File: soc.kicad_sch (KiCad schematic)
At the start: 10 parts, among them U1 STM32MP135AAFx, U2 STM32MP131AAEx, U3 ATSAMA5D21

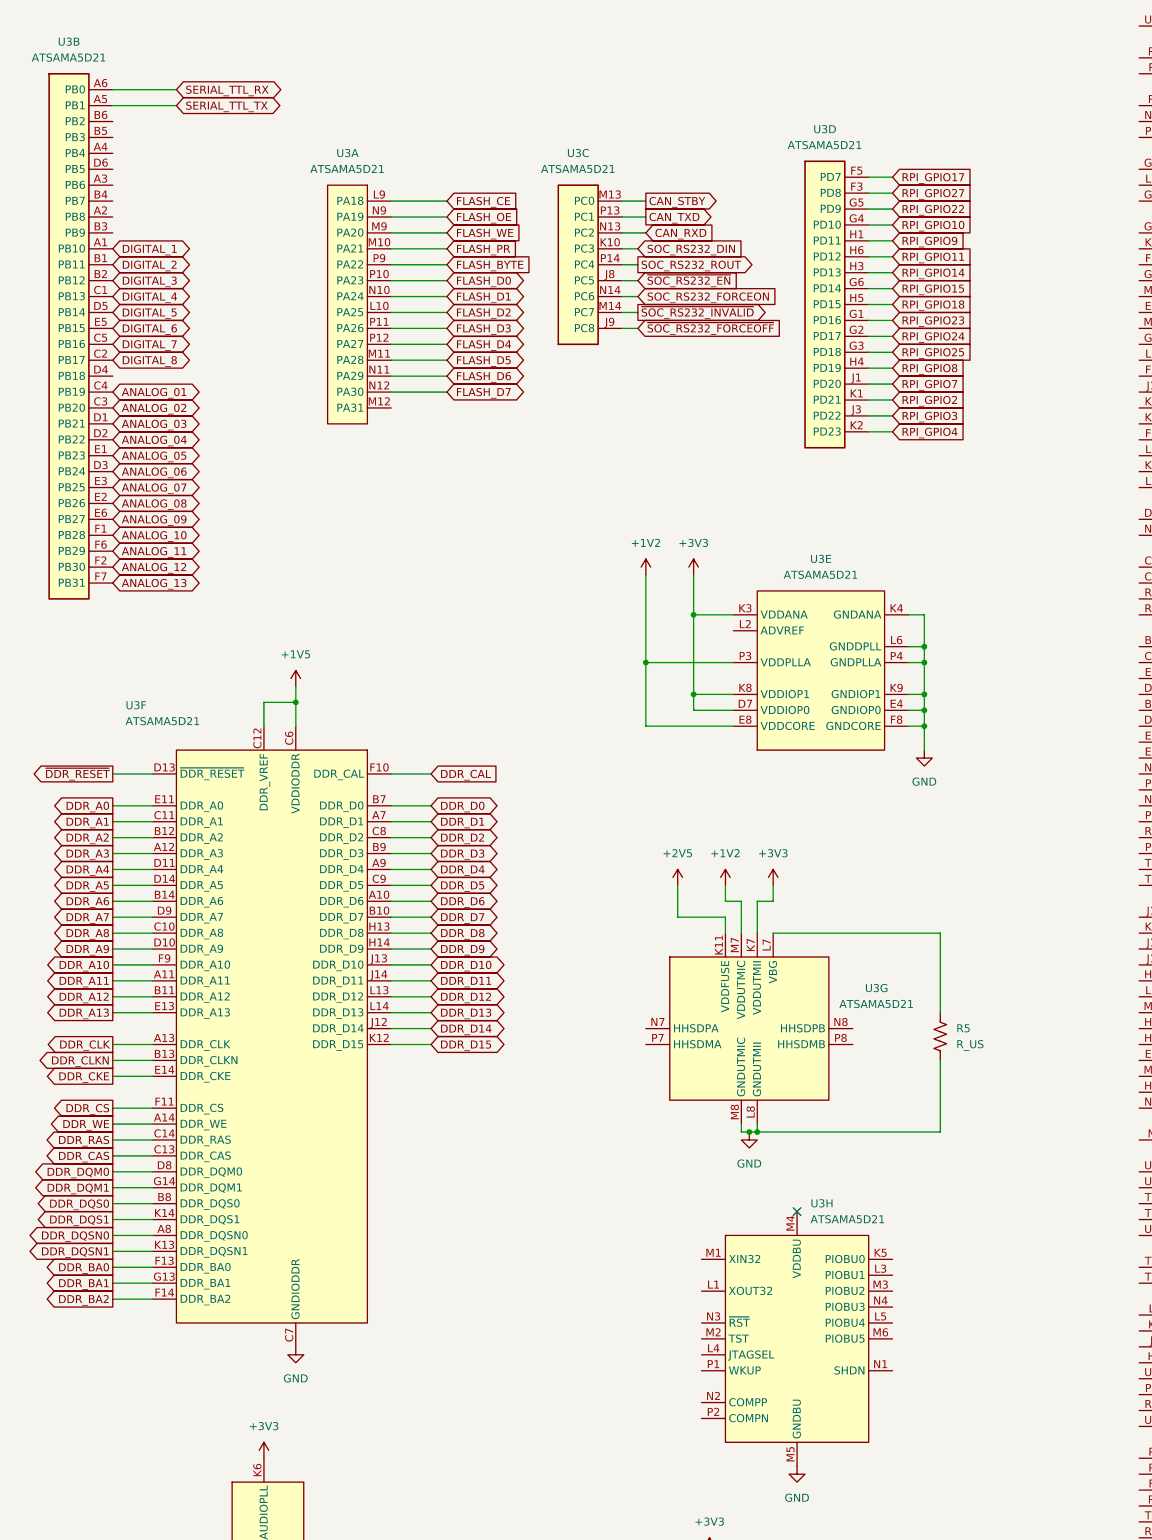
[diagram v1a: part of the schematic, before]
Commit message: before caleb
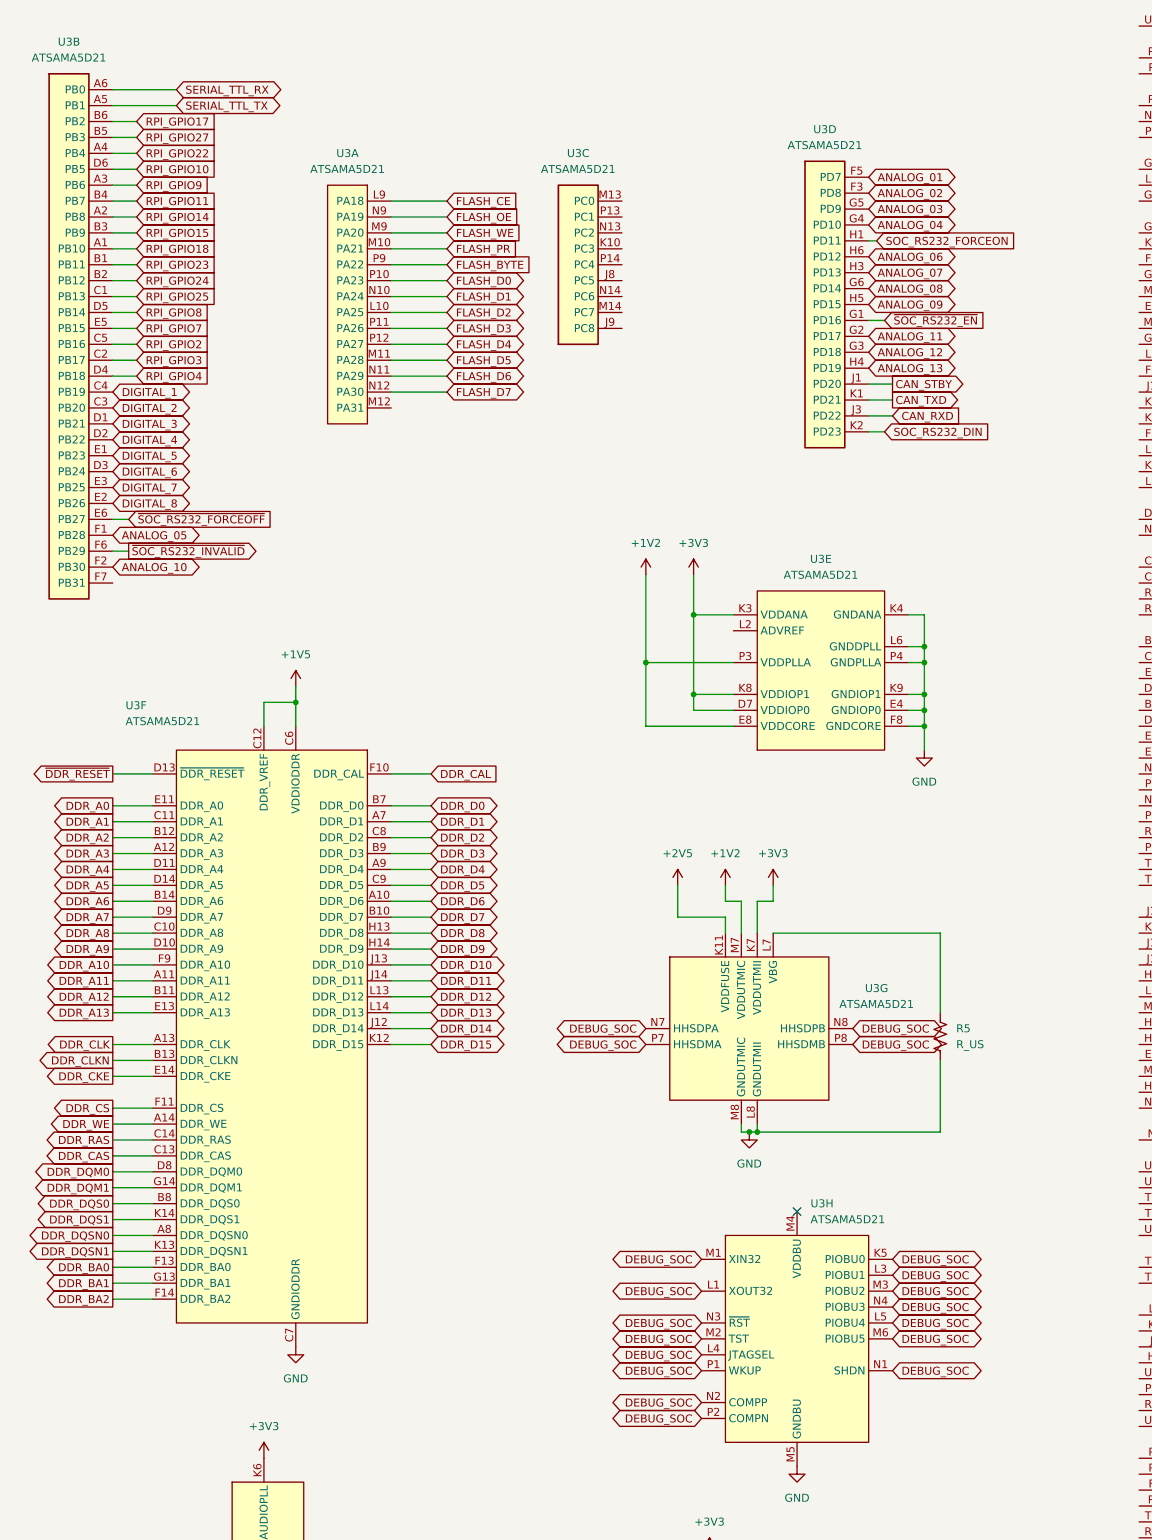
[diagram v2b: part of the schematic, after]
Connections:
- net ANALOG_01: now also U3.F5 (PD7); no longer U3.C4 (PB19)
- net ANALOG_02: now also U3.F3 (PD8); no longer U3.C3 (PB20)
- net ANALOG_03: now also U3.G5 (PD9); no longer U3.D1 (PB21)
- net ANALOG_04: now also U3.G4 (PD10); no longer U3.D2 (PB22)
- net ANALOG_05: now also U3.F1 (PB28); no longer U3.E1 (PB23)
- net ANALOG_06: now also U3.H6 (PD12); no longer U3.D3 (PB24)
- net ANALOG_07: now also U3.H3 (PD13); no longer U3.E3 (PB25)
- net ANALOG_08: now also U3.G6 (PD14); no longer U3.E2 (PB26)
- net ANALOG_09: now also U3.H5 (PD15); no longer U3.E6 (PB27)
- net ANALOG_10: now also U3.F2 (PB30); no longer U3.F1 (PB28)
- net ANALOG_11: now also U3.G2 (PD17); no longer U3.F6 (PB29)
- net ANALOG_12: now also U3.G3 (PD18); no longer U3.F2 (PB30)
- net ANALOG_13: now also U3.H4 (PD19); no longer U3.F7 (PB31)
- net CAN_RXD: now also U3.J3 (PD22); no longer U3.N13 (PC2)
- net CAN_STBY: now also U3.J1 (PD20); no longer U3.M13 (PC0)
- net CAN_TXD: now also U3.K1 (PD21); no longer U3.P13 (PC1)
- net DIGITAL_1: now also U3.C4 (PB19); no longer U3.A1 (PB10)
- net DIGITAL_2: now also U3.C3 (PB20); no longer U3.B1 (PB11)
- net DIGITAL_3: now also U3.D1 (PB21); no longer U3.B2 (PB12)
- net DIGITAL_4: now also U3.D2 (PB22); no longer U3.C1 (PB13)
- net DIGITAL_5: now also U3.E1 (PB23); no longer U3.D5 (PB14)
- net DIGITAL_6: now also U3.D3 (PB24); no longer U3.E5 (PB15)
- net DIGITAL_7: now also U3.E3 (PB25); no longer U3.C5 (PB16)
- net DIGITAL_8: now also U3.E2 (PB26); no longer U3.C2 (PB17)
- net RPI_GPIO10: now also U3.D6 (PB5); no longer U3.G4 (PD10)
- net RPI_GPIO11: now also U3.B4 (PB7); no longer U3.H6 (PD12)
- net RPI_GPIO14: now also U3.A2 (PB8); no longer U3.H3 (PD13)
- net RPI_GPIO15: now also U3.B3 (PB9); no longer U3.G6 (PD14)
- net RPI_GPIO17: now also U3.B6 (PB2); no longer U3.F5 (PD7)
- net RPI_GPIO18: now also U3.A1 (PB10); no longer U3.H5 (PD15)
- net RPI_GPIO2: now also U3.C5 (PB16); no longer U3.K1 (PD21)
- net RPI_GPIO22: now also U3.A4 (PB4); no longer U3.G5 (PD9)
- net RPI_GPIO23: now also U3.B1 (PB11); no longer U3.G1 (PD16)
- net RPI_GPIO24: now also U3.B2 (PB12); no longer U3.G2 (PD17)
- net RPI_GPIO25: now also U3.C1 (PB13); no longer U3.G3 (PD18)
- net RPI_GPIO27: now also U3.B5 (PB3); no longer U3.F3 (PD8)
- net RPI_GPIO3: now also U3.C2 (PB17); no longer U3.J3 (PD22)
- net RPI_GPIO4: now also U3.D4 (PB18); no longer U3.K2 (PD23)
- net RPI_GPIO7: now also U3.E5 (PB15); no longer U3.J1 (PD20)
- net RPI_GPIO8: now also U3.D5 (PB14); no longer U3.H4 (PD19)
- net RPI_GPIO9: now also U3.A3 (PB6); no longer U3.H1 (PD11)
- net SOC_RS232_DIN: now also U3.K2 (PD23); no longer U3.K10 (PC3)
- net SOC_RS232_FORCEON: now also U3.H1 (PD11); no longer U3.N14 (PC6)
- net ~{SOC_RS232_EN}: now also U3.G1 (PD16); no longer U3.J8 (PC5)
- net ~{SOC_RS232_FORCEOFF}: now also U3.E6 (PB27); no longer U3.J9 (PC8)
- net ~{SOC_RS232_INVALID}: now also U3.F6 (PB29); no longer U3.M14 (PC7)
- net DEBUG_SOC: now reaches U3.N7 (HHSDPA)
- net DEBUG_SOC: now also U3.K5 (PIOBU0), U3.L1 (XOUT32), U3.L3 (PIOBU1), U3.L4 (JTAGSEL), U3.L5 (PIOBU4), U3.M1 (XIN32), U3.M2 (TST), U3.M3 (PIOBU2), U3.M6 (PIOBU5), U3.N1 (SHDN), U3.N2 (COMPP), U3.N3 (~{RST}), U3.N4 (PIOBU3), U3.N8 (HHSDPB), U3.P1 (WKUP), U3.P2 (COMPN), U3.P7 (HHSDMA), U3.P8 (HHSDMB)
- net SOC_RS232_ROUT: no longer names the net of U3.P14 (PC4)

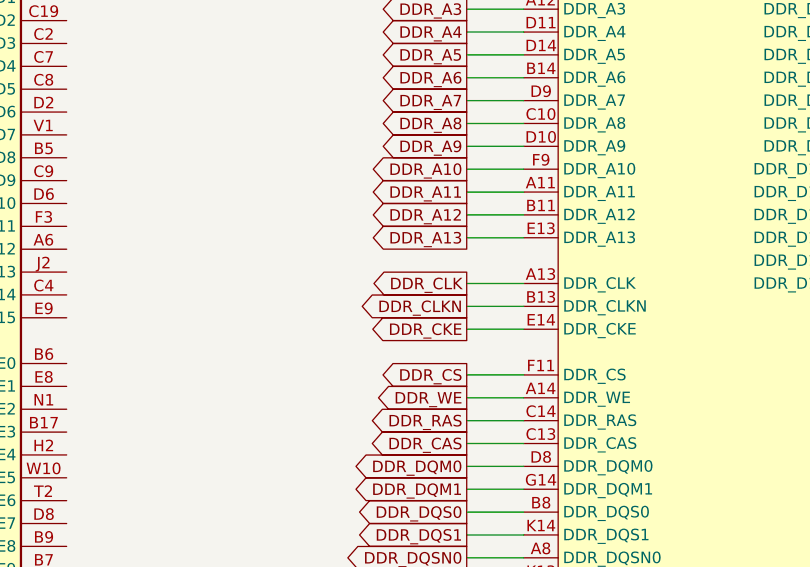
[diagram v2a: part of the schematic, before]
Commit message: after rough draft submission
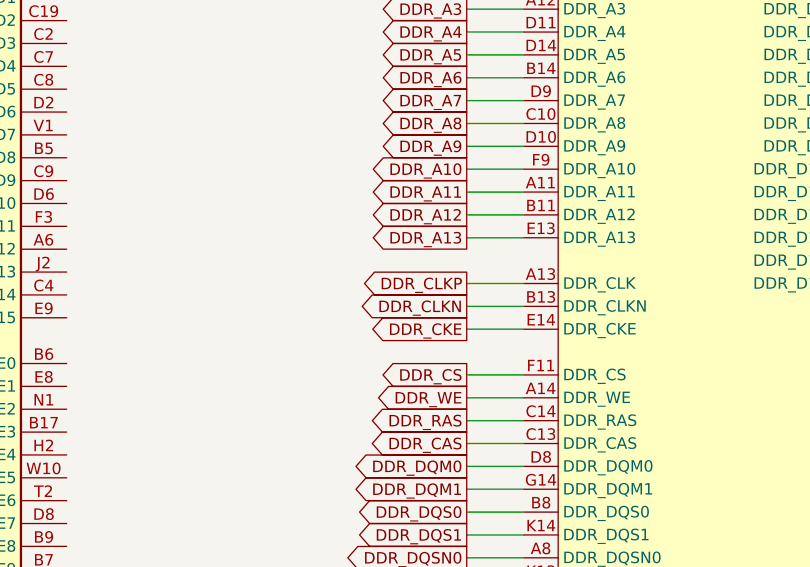
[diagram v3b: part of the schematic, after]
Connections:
- net DDR_CLK renamed DDR_CLKP
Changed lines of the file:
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@@
 		)
 	)
-	(global_label "DDR_CLK"
+	(global_label "DDR_CLKP"
 		(shape output)
 		(at 250.19 215.9 180)
